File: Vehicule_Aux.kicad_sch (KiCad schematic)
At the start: 25 parts, among them Q43 IRLZ44N, Q66 2N7000, Q67 2N7000, SW10 TH_Aux, U11 LM339

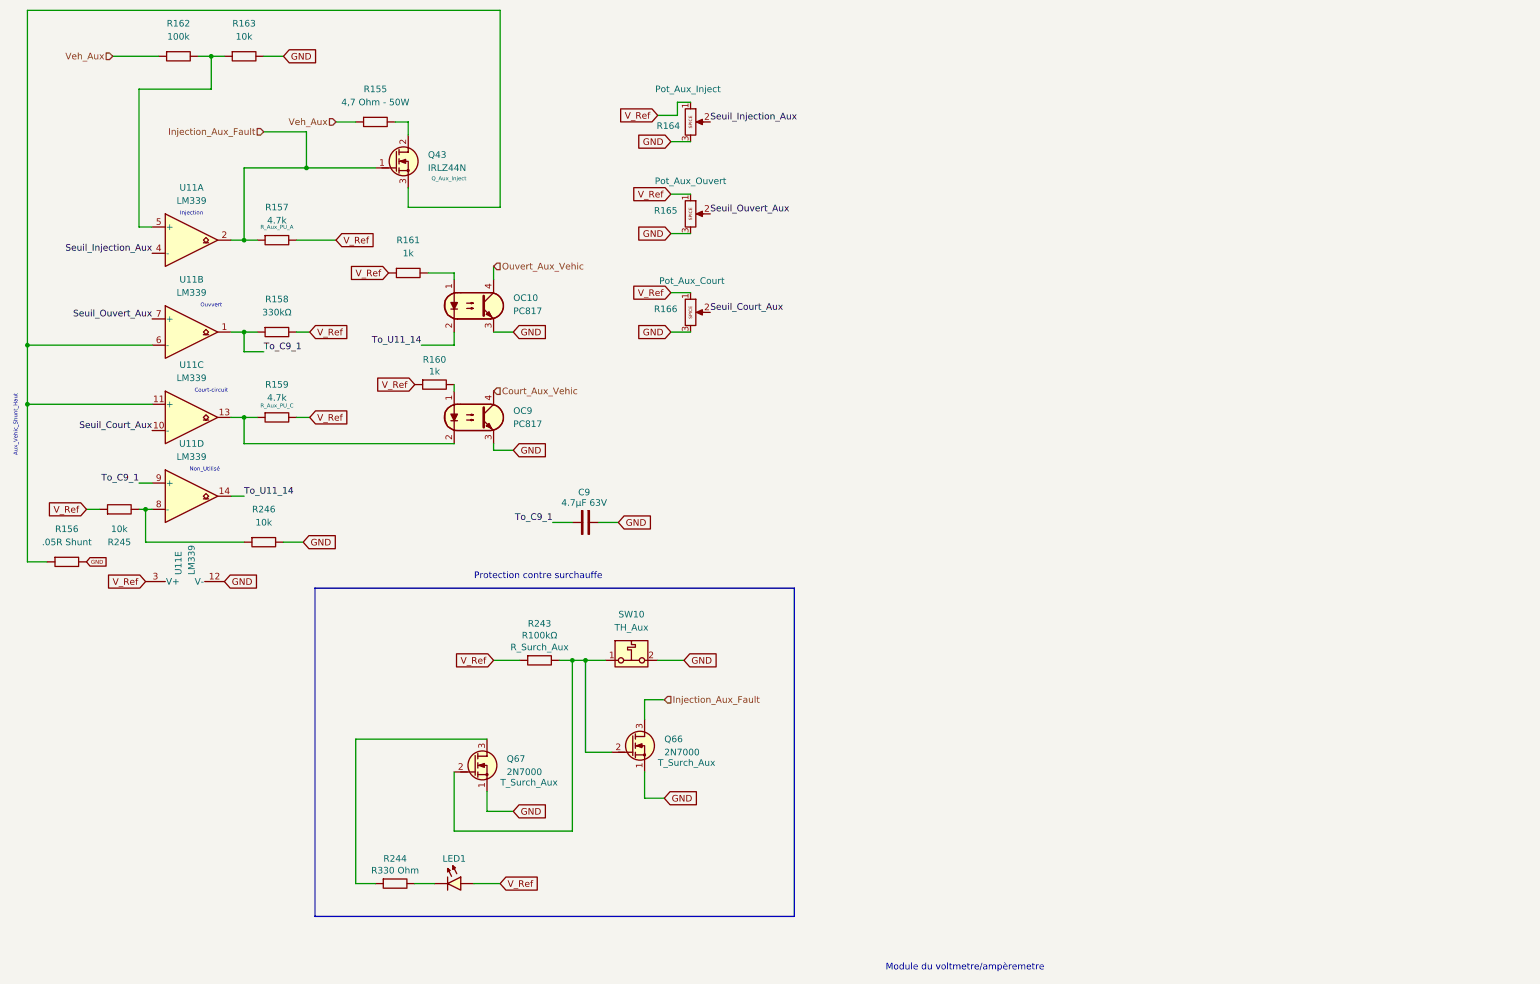
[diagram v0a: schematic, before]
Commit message: Add files via upload
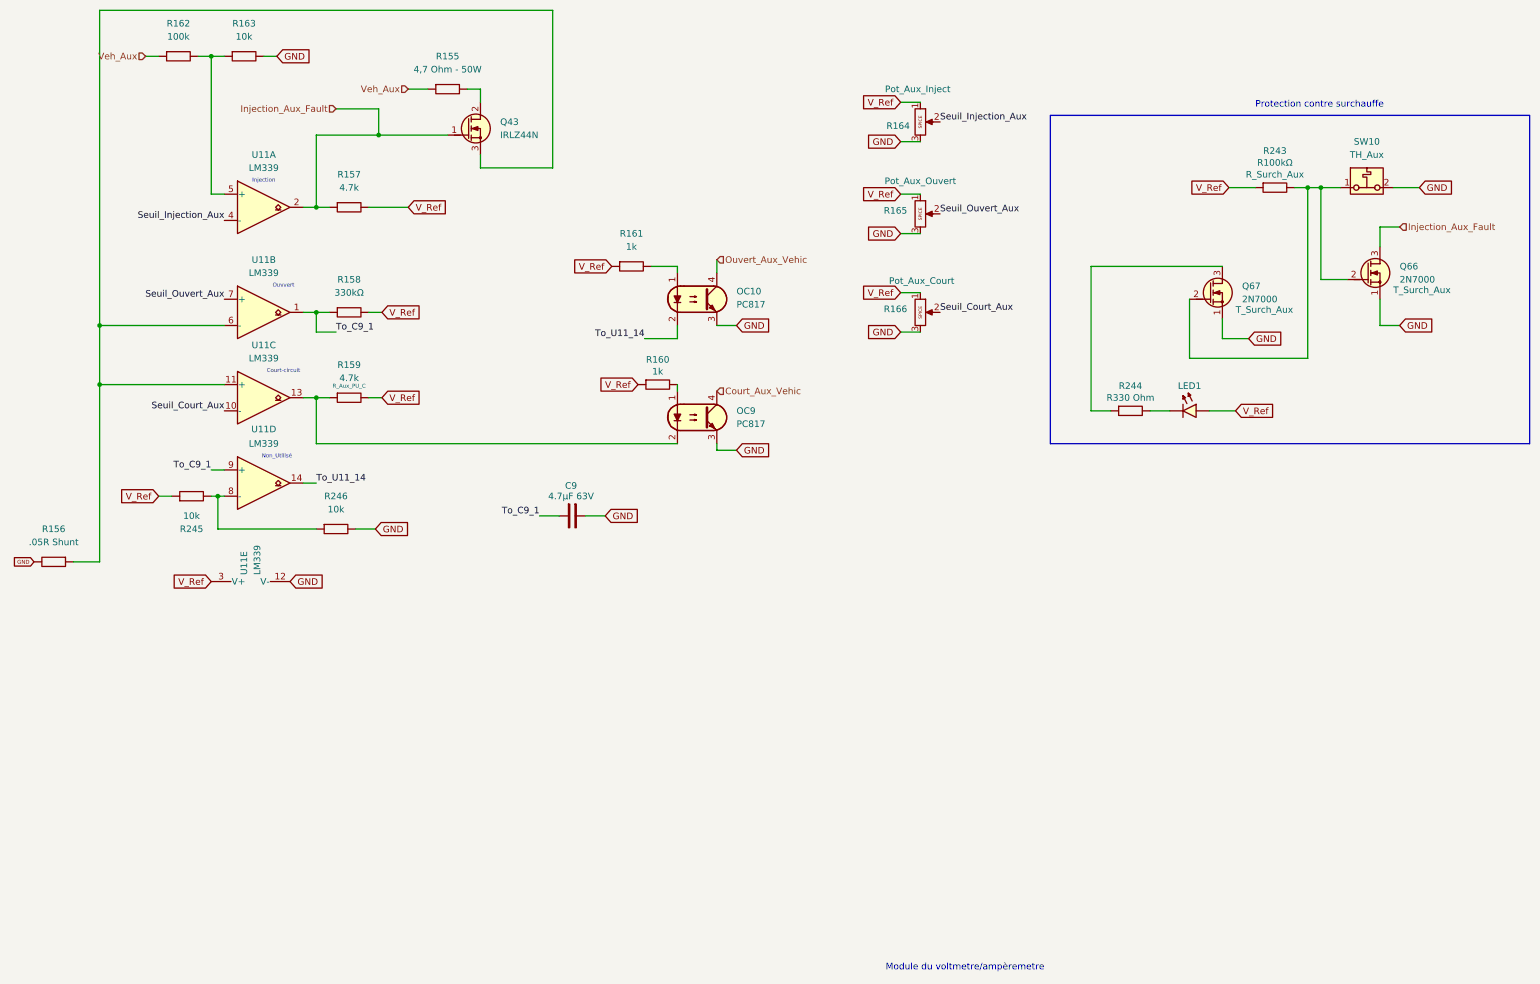
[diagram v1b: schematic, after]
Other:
- note removed: "Aux_Vehic_Shunt_Haut"
- moved on the sheet: C9, LED1, OC10, OC9, Q43, Q66, Q67, R155, R156, R157, R158, R159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
